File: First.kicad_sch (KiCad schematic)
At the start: 48 parts, among them J1 UART0, J2 UART1, J3 USB_B_Micro, J4 UART2, J5 UART3, U1 CP2102N-DEV0, U2 TUSB2046IBVFR, U3 CP2102N-DEV1, U4 CP2102N_DEV2, U5 LD1086V33-DG, U6 CP2102N-A01-GQFN24, Y1 HC49SDLF-8.00MHz

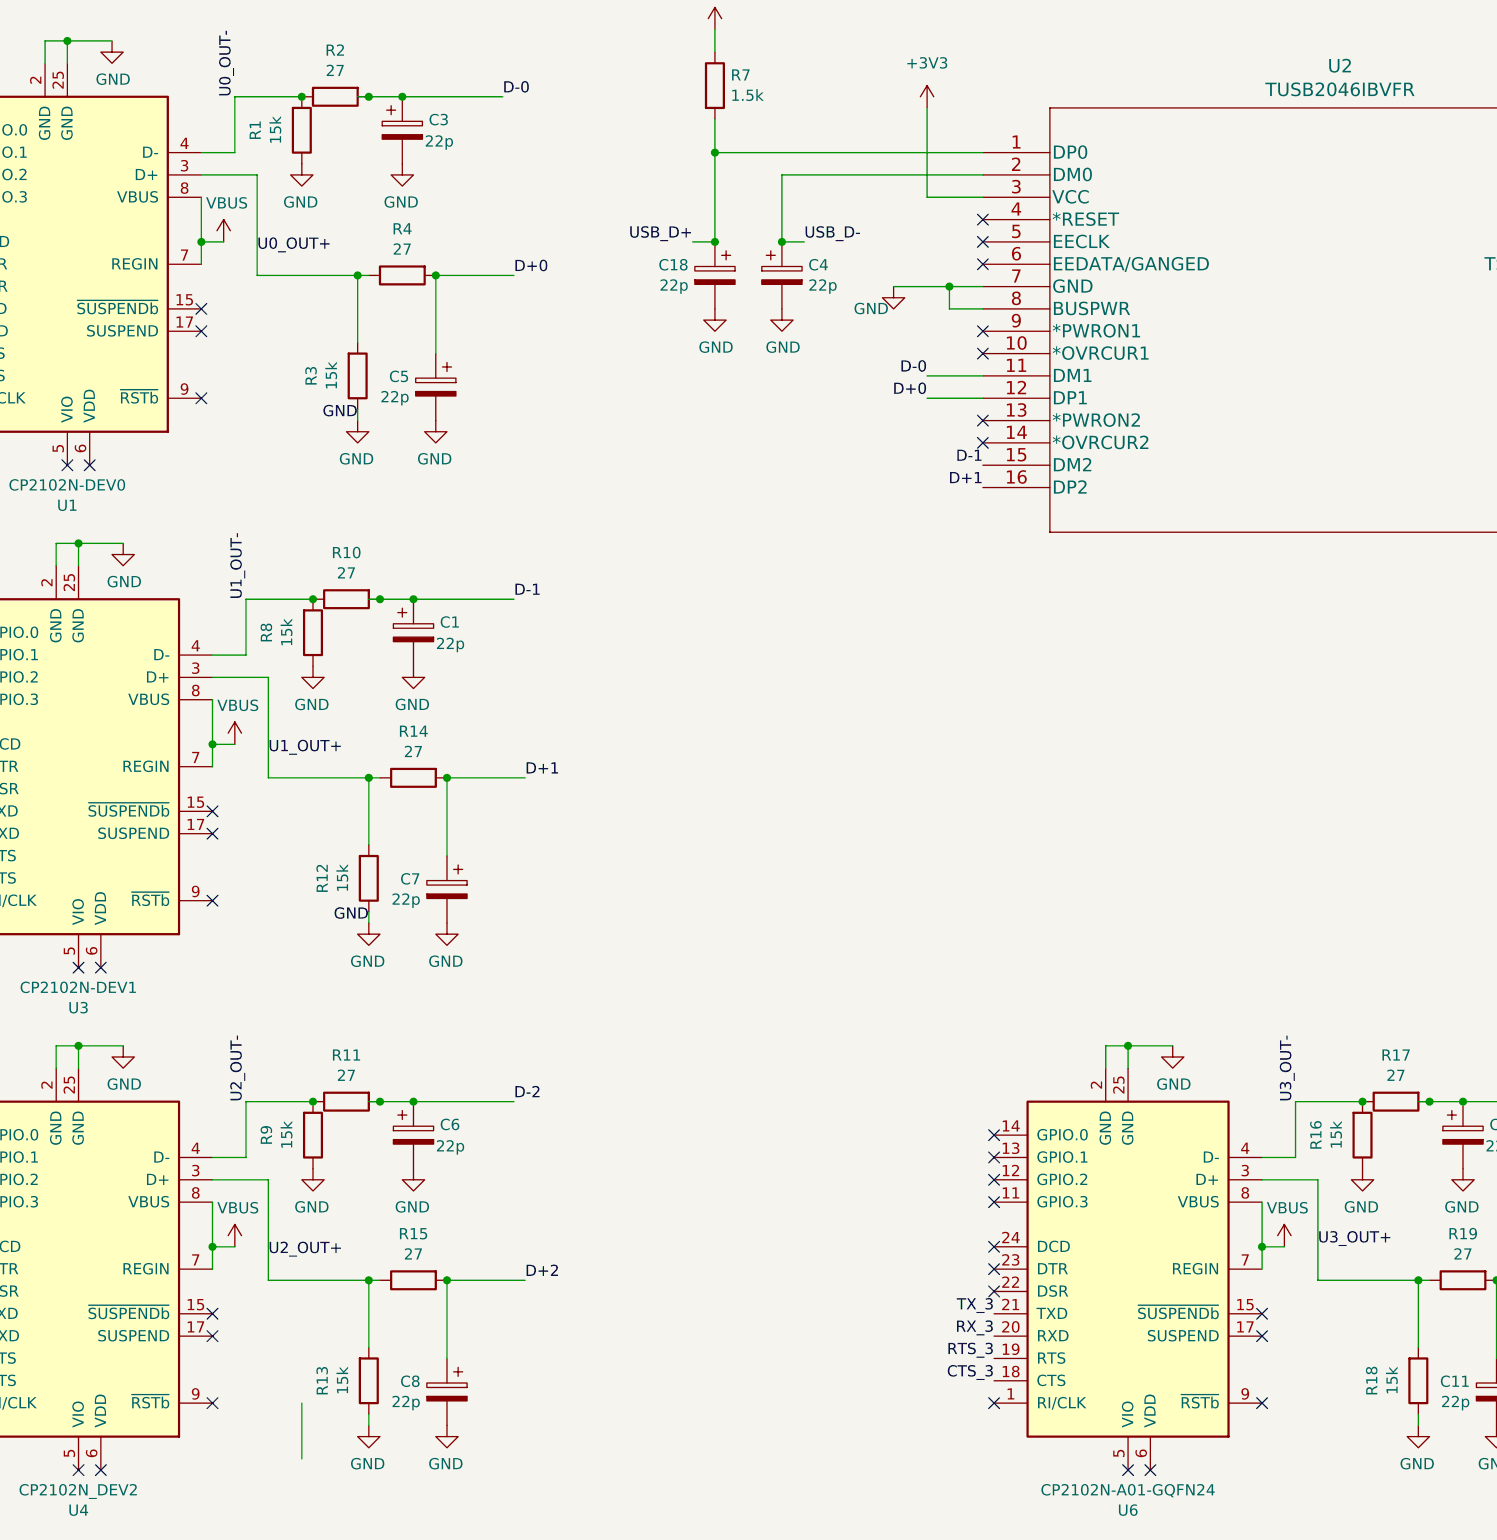
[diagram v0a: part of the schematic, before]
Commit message: Ordered version
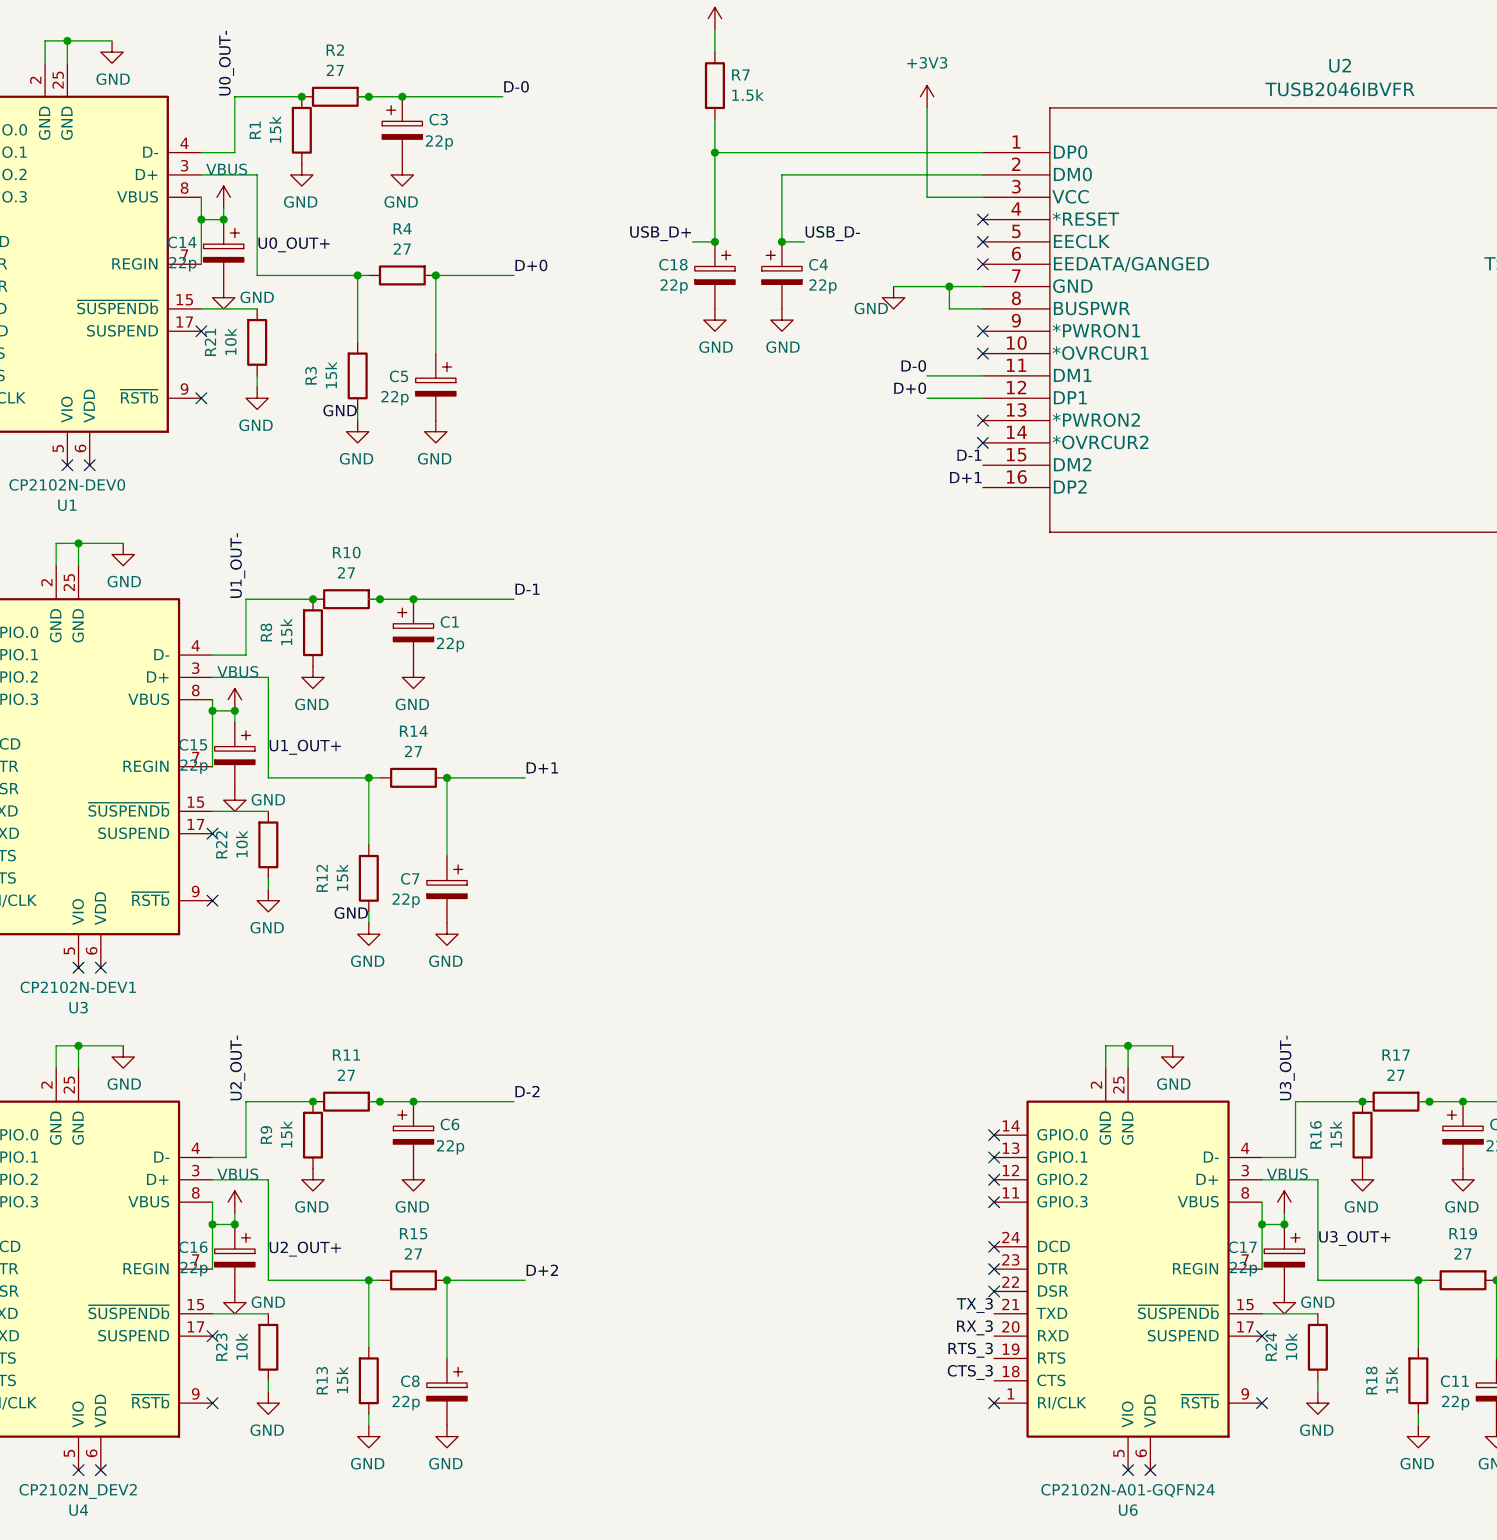
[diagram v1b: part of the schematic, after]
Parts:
- added C14, C15, C16, C17: 22p, Capacitor_SMD:C_0603_1608Metric, symbol First-rescue:CP-Device
- added R21, R22, R23, R24: 10k, Resistor_SMD:R_0603_1608Metric, symbol Device:R
- D1: footprint LED_THT:LED_D3.0mm -> LED_SMD:LED_0805_2012Metric
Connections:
- net GND: now also C14.2, C15.2, C16.2, C17.2, R21.1, R22.1, R23.1, R24.1
- net VBUS: now also C14.1, C15.1, C16.1, C17.1
- net at U1.15 (~{SUSPENDb}): now also R21.2
- net at U3.15 (~{SUSPENDb}): now also R22.2
- net at U6.15 (~{SUSPENDb}): now also R24.2
- net at U4.15 (~{SUSPENDb}): now also R23.2
- no-connect marks 65 -> 61
